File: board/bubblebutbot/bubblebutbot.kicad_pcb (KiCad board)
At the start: 2 copper layers, 90 x 30 mm, 69 parts, among them J1 JST XH, J10 JST XH, J11 JST XH, J13 JST XH, J2 USB_C_Receptacle, J3 Conn_01x03_Socket, J4 Conn_01x03_Socket, J5 Conn_01x03_Socket, J6 Conn_01x03_Socket, J7 Conn_01x03_Socket, J8 Conn_01x03_Socket, J9 JST XH, Q1 FDN336P, U1 DRV8833PWP, U2 ESP32-S3-WROOM-1, U3 AP2112K-3.3, U4 LIS3DH

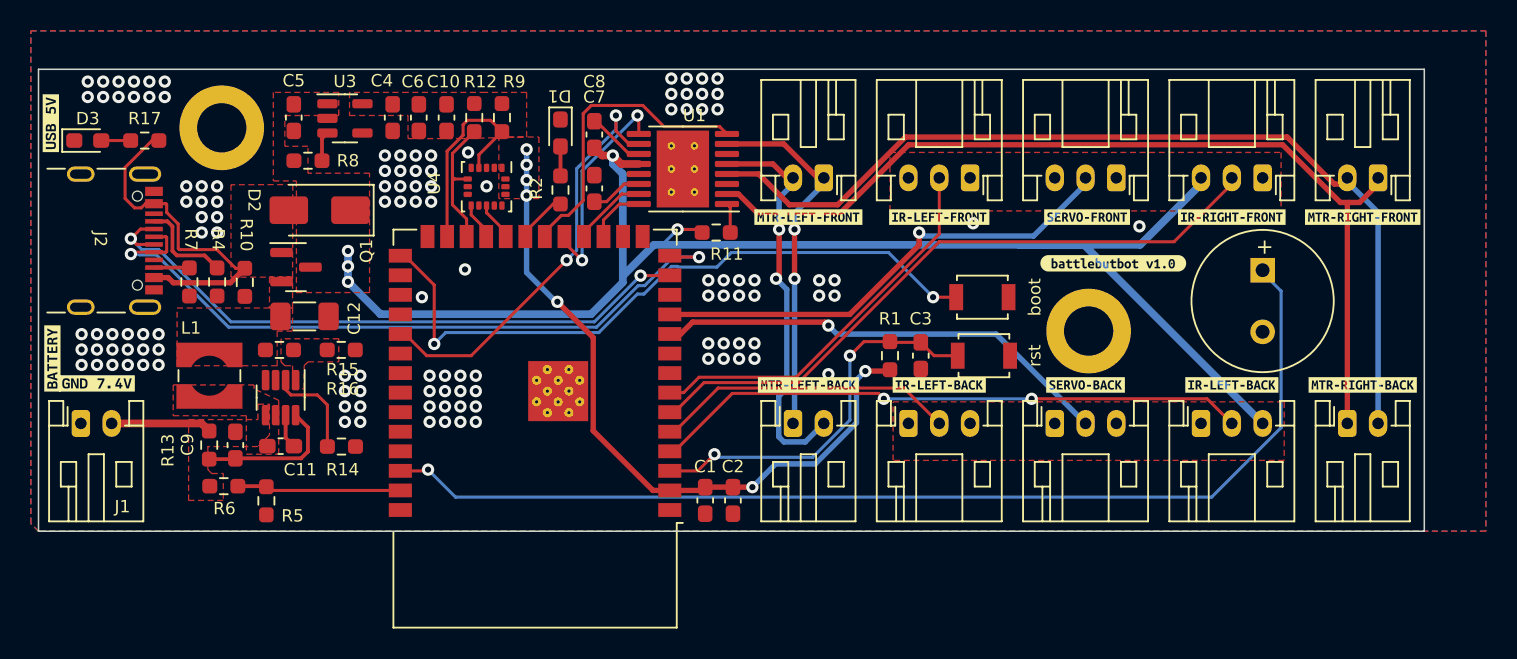
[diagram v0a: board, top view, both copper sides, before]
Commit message: pcb 1v04
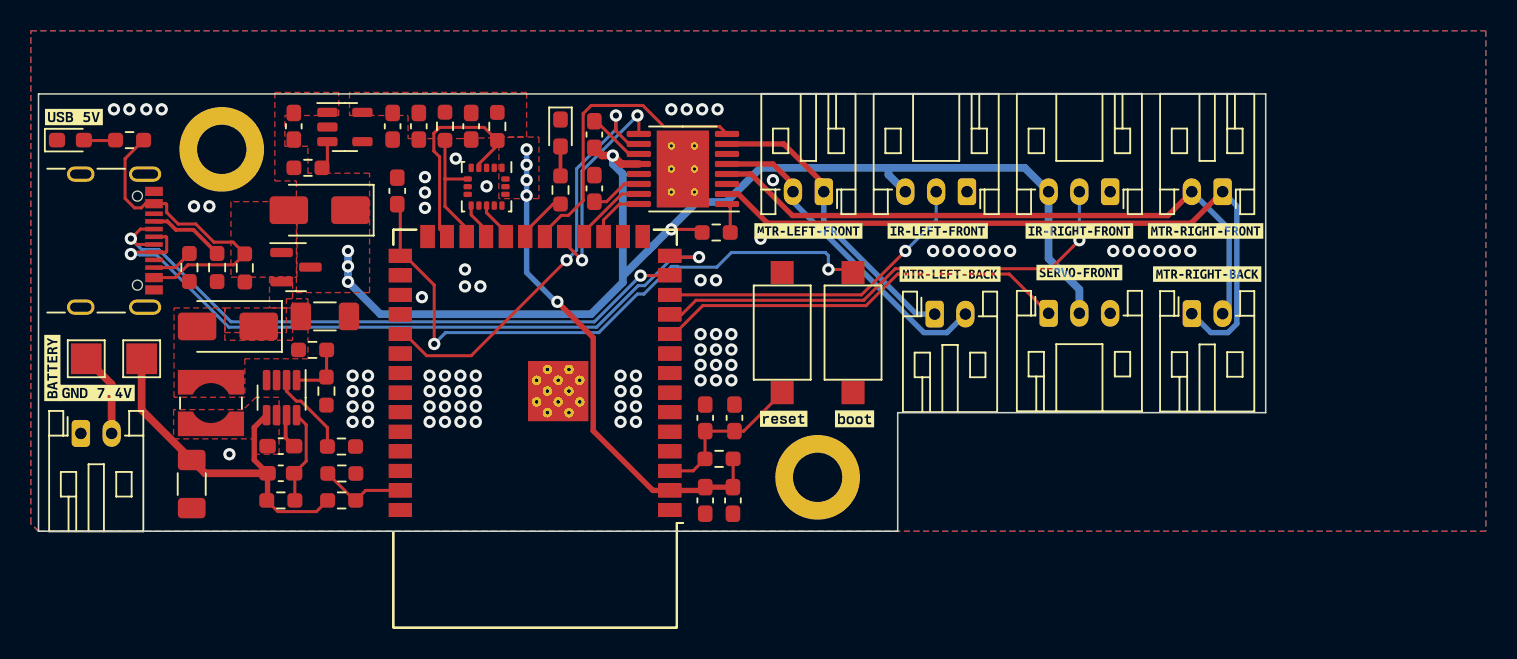
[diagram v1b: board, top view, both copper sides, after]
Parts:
- removed BZ1: Buzzer, Buzzer_Beeper:MagneticBuzzer_PUI_AT-0927-TT-6-R
- removed J8: Conn_01x03_Socket, Connector_JST:JST_PH_S3B-PH-K_1x03_P2.00mm_Horizontal
- removed R13: 5.1K, Resistor_SMD:R_0603_1608Metric_Pad0.98x0.95mm_HandSolder
- removed boot, rst: SW_Push, Button_Switch_SMD:SW_SPST_B3U-1000P
- removed kibuzzard-6507382A: G***, kibuzzard-6507382A
- removed kibuzzard-6507384E: G***, kibuzzard-6507384E
- removed kibuzzard-6507385B: G***, kibuzzard-6507385B
- added C13: 1u, Capacitor_SMD:C_0603_1608Metric_Pad1.08x0.95mm_HandSolder, F.Cu at (110.7, 46.6)
- added C14: 0.1uF/50V, Capacitor_SMD:C_0603_1608Metric_Pad1.08x0.95mm_HandSolder, F.Cu at (88.8, 31.9)
- added C16: 22u, Capacitor_SMD:C_1206_3216Metric_Pad1.33x1.80mm_HandSolder, F.Cu at (75.5, 50.9)
- added D4: SS14, Diode_SMD:D_SMA, F.Cu at (77.8, 40.7)
- added R3: 100k, Resistor_SMD:R_0603_1608Metric_Pad0.98x0.95mm_HandSolder, F.Cu at (81.2, 52.0)
- added SW1: SW_Push, Button_Switch_SMD:SW_SPST_CK_RS282G05A3, F.Cu at (113.8, 41.1)
- added SW2: SW_Push, Button_Switch_SMD:SW_SPST_CK_RS282G05A3, F.Cu at (118.4, 41.1)
- added U2: ESP32-S3-WROOM-1, RF_Module:ESP32-S3-WROOM-1, F.Cu at (97.8, 47.4)
- added kibuzzard-65510192: G***, kibuzzard-65510192, F.Cu at (118.5, 46.7)
- added kibuzzard-655101A0: G***, kibuzzard-655101A0, F.Cu at (113.9, 46.7)
- C11: value 100n -> 10n
- C3: value 10u -> 0.1uF/50V
- J5, J6: value Conn_01x03_Socket -> Conn_01x01_Pin; footprint Connector_JST:JST_PH_S3B-PH-K_1x03_P2.00mm_Horizontal -> TestPoint:TestPoint_Pad_2.0x2.0mm
- R11: value 50k -> 100k
- R16: value R -> 12k
- U5: value ~ -> SY8303
- kibuzzard-650738AB: moved to B.Cu
- moved J6 68.9 mm to (72.2, 42.8)
- moved kibuzzard-650738AB 65.4 mm to (71.5, 51.0), turned to 180 degrees
- moved J5 53.6 mm to (68.6, 42.8)
- moved H2 20.0 mm to (116.1, 50.5)
- moved C3 14.6 mm to (108.8, 46.6), turned to 90 degrees
- moved R1 13.0 mm to (109.7, 49.3), turned to 180 degrees
- moved kibuzzard-65073881 12.4 mm to (141.4, 37.3)
- moved J9 12.4 mm to (140.4, 39.9)
- moved kibuzzard-65073819 11.7 mm to (124.7, 37.3)
- moved J11 11.6 mm to (123.7, 39.9)
- moved kibuzzard-65073803 10.2 mm to (141.3, 34.5)
- moved J13 10.1 mm to (142.4, 31.9)
- moved J4 9.94 mm to (135.1, 31.9)
- moved kibuzzard-650737FA 9.94 mm to (133.1, 34.5)
- moved J7 9.84 mm to (131.1, 39.9), turned to 0 degrees
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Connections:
- C12 pad 1: 5V_BAT -> Net-(D4-A)
- C9 pad 1: +7.5V -> BAT_OUT
- J5 pad 1: GND -> +7.5V
- J6 pad 1: GND -> BAT_OUT
- J7 pad 1: GND -> ESP32-SRV-F
- J7 pad 2: ESP32-SRV-F -> +5V
- J7 pad 3: +5V -> GND
- L1 pad 2: 5V_BAT -> Net-(D4-A)
- R11 pad 1: +5V -> Net-(U1-nSLEEP)
- R11 pad 2: Net-(U1-nSLEEP) -> +5V
- R15 pad 2: 5V_BAT -> Net-(D4-A)
- R6 pad 2: +7.5V -> BAT_OUT
- U2 pad 10: ESP32-SRV-B -> ESP32-SRV-F
- U2 pad 11: ESP32-SRV-F -> ESP32-IR-FR
- U2 pad 12: unconnected-(U2-GPIO8/TOUCH8/ADC1_CH7/SUBSPICS1-Pad12) -> ESP32-IR-FL
- U2 pad 38: ESP32-BUZZER -> unconnected-(U2-GPIO2/TOUCH2/ADC1_CH1-Pad38)
- U2 pad 4: ESP32-IR-BR -> unconnected-(U2-GPIO4/TOUCH4/ADC1_CH3-Pad4)
- U2 pad 5: ESP32-IR-BL -> unconnected-(U2-GPIO5/TOUCH5/ADC1_CH4-Pad5)
- U2 pad 6: ESP32-IR-FR -> unconnected-(U2-GPIO6/TOUCH6/ADC1_CH5-Pad6)
- U2 pad 7: ESP32-IR-FL -> unconnected-(U2-GPIO7/TOUCH7/ADC1_CH6-Pad7)
- U5 pad 5: +7.5V -> BAT_OUT
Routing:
- net ESP32-BUZZER: track 70.4 -> 0.00 mm, vias 1 -> 0
- net ESP32-IR-BR: track 38.9 -> 0.00 mm, vias 2 -> 0
- net ESP32-SRV-B: track 30.0 -> 0.00 mm, vias 1 -> 0
- net BAT_OUT: track 0.00 -> 24.0 mm
- net +5V: track 97.7 -> 78.0 mm
- net ESP32-IR-BL: track 19.6 -> 0.00 mm
- net MOTOR-RIGHT-BR: track 60.7 -> 41.0 mm
- net ESP32-RESET: track 25.1 -> 10.5 mm, vias 2 -> 0
- net MOTOR-RIGHT-BL: track 61.0 -> 46.5 mm
- net +3.3V: track 45.9 -> 32.7 mm, vias 7 -> 5
- net ESP32-IR-FR: track 42.6 -> 31.7 mm, vias 0 -> 1
- net ESP32-BATTERY-READ: track 10.7 -> 5.71 mm
- net MOTOR-LEFT-BR: track 25.8 -> 21.2 mm, vias 2 -> 0
- net MOTOR-LEFT-BL: track 23.7 -> 19.5 mm, vias 2 -> 0
- net ESP32-SRV-F: track 31.2 -> 27.3 mm, vias 1 -> 0
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- added copper zone on F.Cu, net Net-(D4-A)
- removed copper zone on F.Cu, net +7.5V
- removed copper zone on F.Cu, net Net-(U5-FB)
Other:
- board size 90 x 30 mm -> 79.7 x 28.4 mm

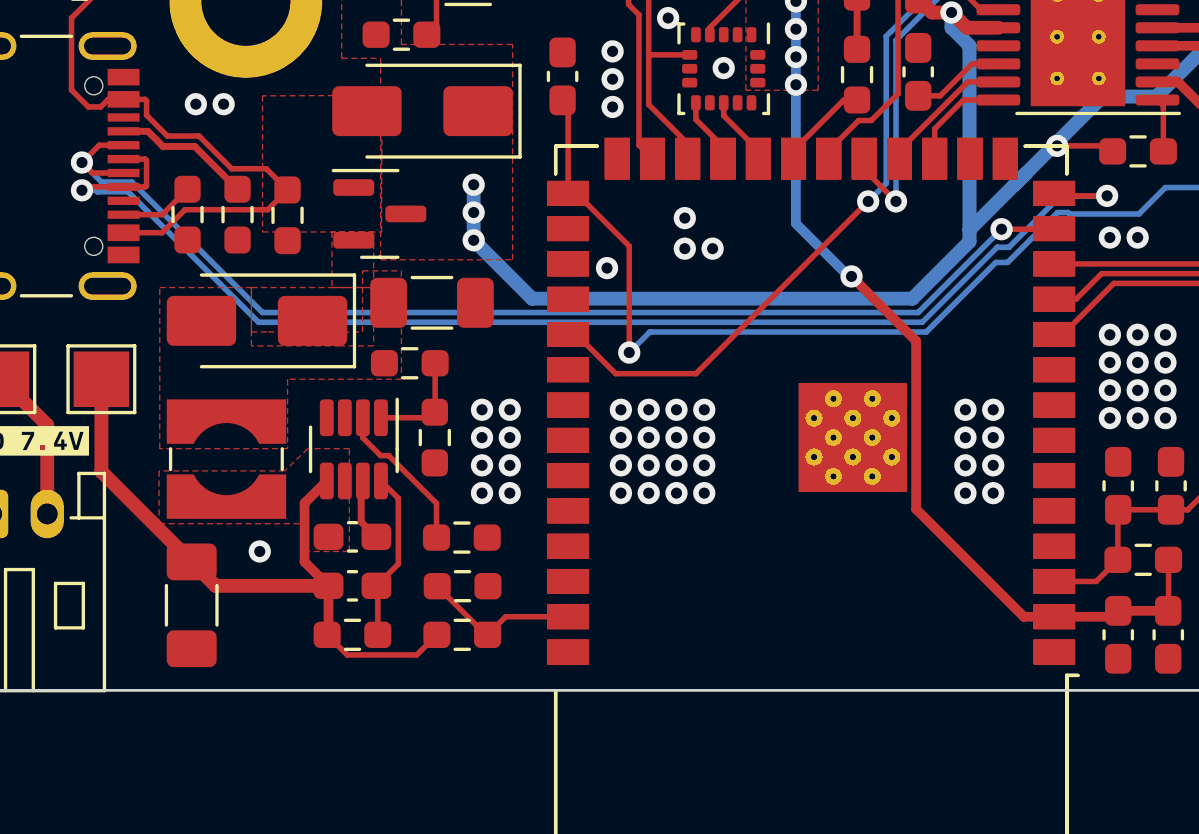
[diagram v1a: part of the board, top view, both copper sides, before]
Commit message: small fix
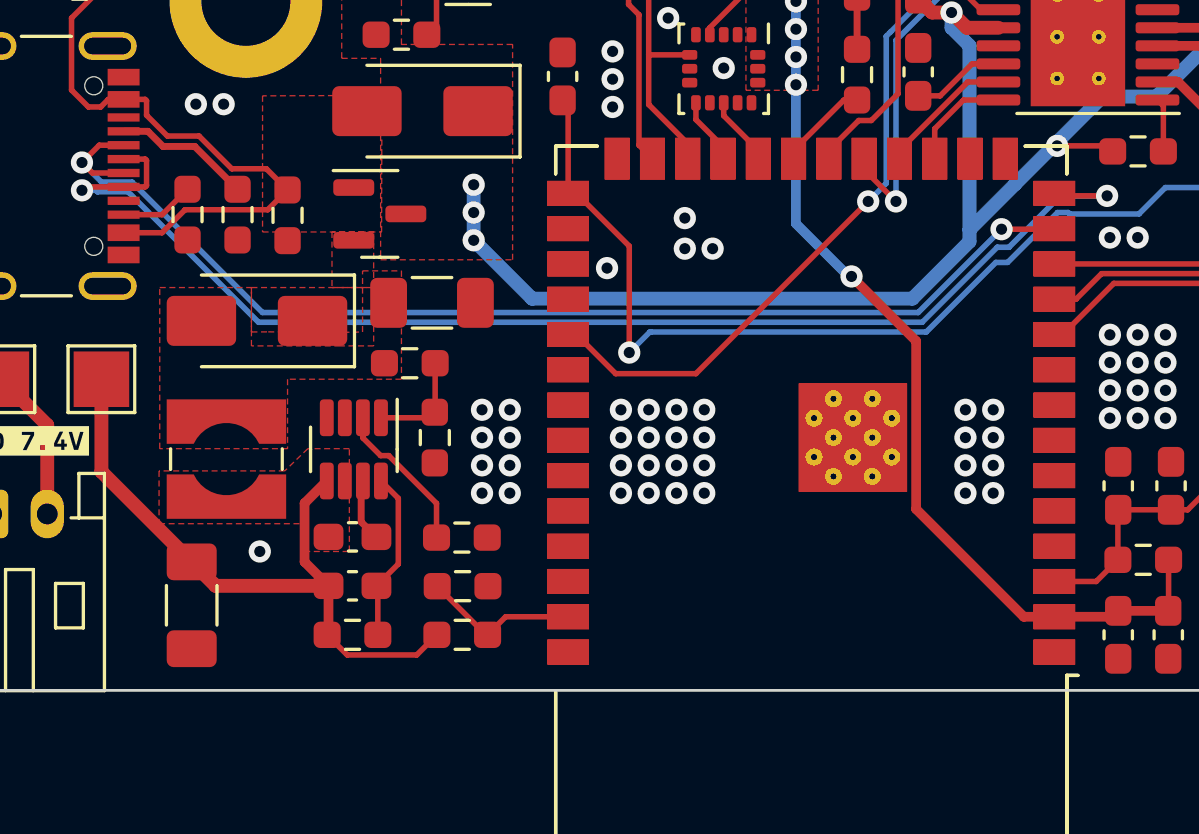
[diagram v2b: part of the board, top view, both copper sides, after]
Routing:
- net +5V: track 78.0 -> 77.4 mm
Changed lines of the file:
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@@
     (fp_line (start 1.6 0.8) (end -1.6 0.8)
       (stroke (width 0.1) (type solid)) (layer "F.Fab"))
-    (pad "1" smd roundrect locked (at -1.5625 0 270) (size 1.325 1.8) (layers "F.Cu" "F.Paste" "F.Mask") (roundrect_rratio 0.188679)
+    (pad "1" smd roundrect locked (at -1.5625 0 270) (size 1.325 1.8) (layers "F.Cu" "F.Paste" "F.Mask") (roundrect_rratio 0.1886792453)
       (net 1 "BAT_OUT") (pintype "passive"))
-    (pad "2" smd roundrect locked (at 1.5625 0 270) (size 1.325 1.8) (layers "F.Cu" "F.Paste" "F.Mask") (roundrect_rratio 0.188679)
+    (pad "2" smd roundrect locked (at 1.5625 0 270) (size 1.325 1.8) (layers "F.Cu" "F.Paste" "F.Mask") (roundrect_rratio 0.1886792453)
       (net 2 "GND") (pintype "passive"))
     (model "${KICAD6_3DMODEL_DIR}/Capacitor_SMD.3dshapes/C_1206_3216Metric.wrl"
@@
   (segment (start 110.175 32.625) (end 112.4 30.4) (width 0.5) (layer "B.Cu") (net 5))
   (segment (start 131.1 36.3) (end 133.1 38.3) (width 0.5) (layer "B.Cu") (net 5))
-  (segment (start 105.084314 35.784314) (end 105.468629 35.4) (width 0.5) (layer "B.Cu") (net 5))
   (segment locked (start 85.6 37.8) (end 85.6 35.8) (width 0.5) (layer "B.Cu") (net 5))
   (segment (start 112.4 30.4) (end 120.7 30.4) (width 0.5) (layer "B.Cu") (net 5))
